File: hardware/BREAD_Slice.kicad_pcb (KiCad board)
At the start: 2 copper layers, 72.6 x 100 mm, 16 parts, among them J1 Conn_01x10_Female, J2 I2C_01x04

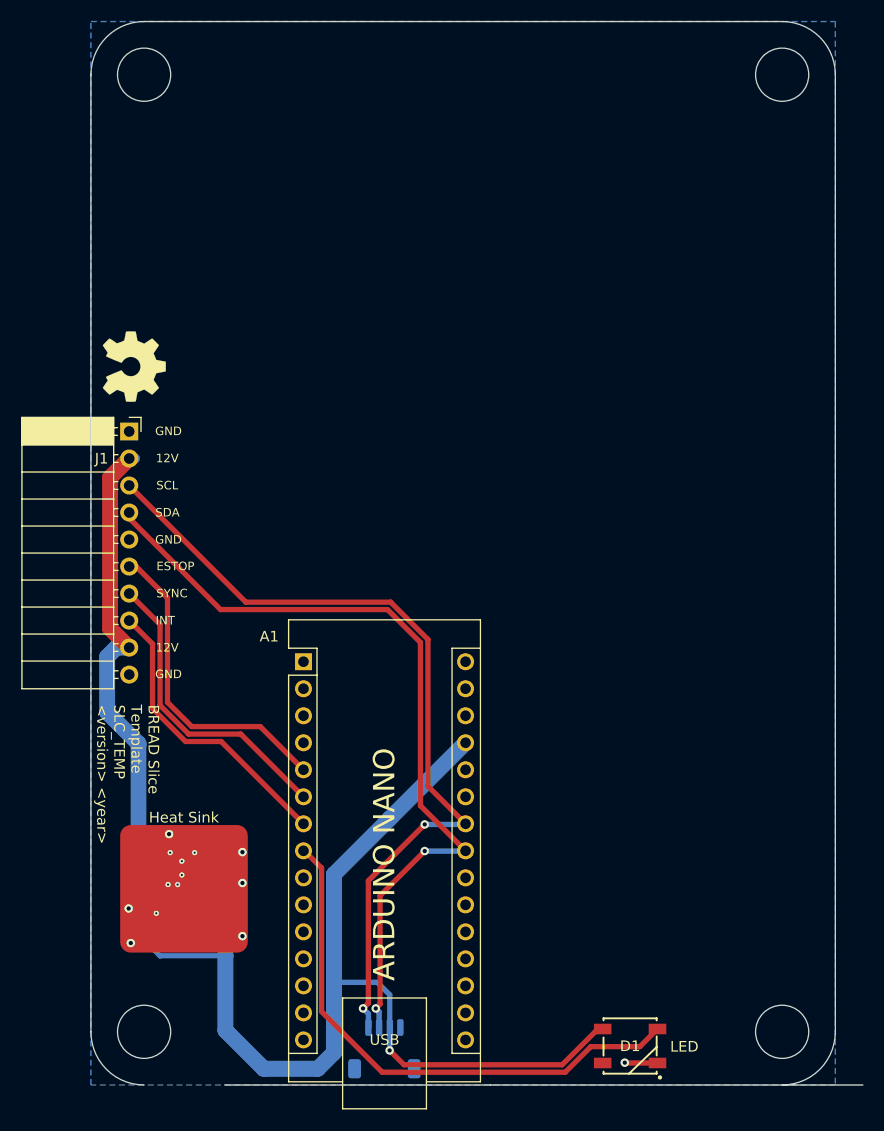
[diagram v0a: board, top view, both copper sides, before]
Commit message: Initial commit
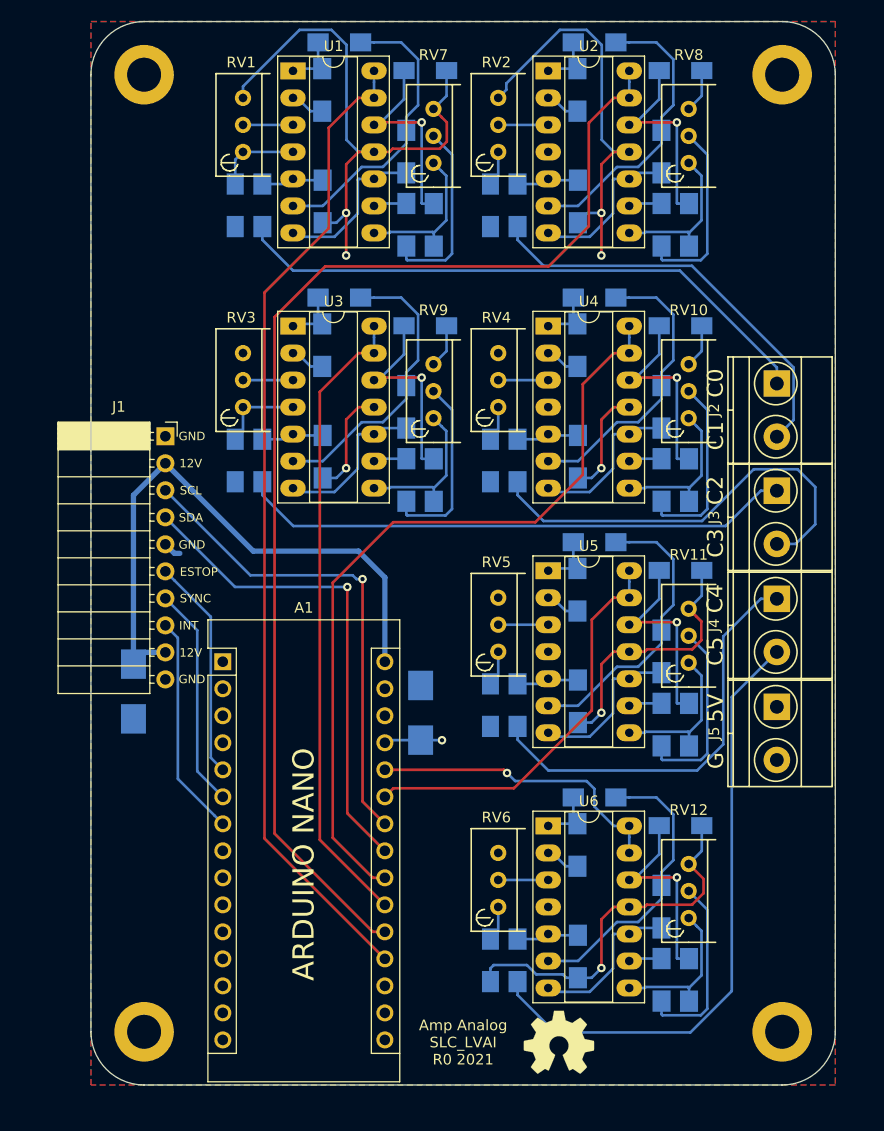
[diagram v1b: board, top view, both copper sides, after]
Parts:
- removed D1: WS2812B_5050, SparkFun-LED:WS2812-5050-4PIN
- removed HS1: Heatsink_Pad, SparkFun-Fuse:Thermal Pad
- removed L1: 4.7uH, Inductor_SMD:L_1210_3225Metric
- added C10: 1uF_t, OCI_UPL_FOOTPRINTS:C_1206_HandSoldering, B.Cu at (178.0, 44.4)
- added C11: 1uF_t, OCI_UPL_FOOTPRINTS:C_1206_HandSoldering, B.Cu at (154.0, 68.4)
- added C12: 1uF_t, OCI_UPL_FOOTPRINTS:C_1206_HandSoldering, B.Cu at (178.0, 68.4)
- added C13: 1uF_t, OCI_UPL_FOOTPRINTS:C_1206_HandSoldering, B.Cu at (178.0, 91.4)
- added C14: 1uF_t, OCI_UPL_FOOTPRINTS:C_1206_HandSoldering, B.Cu at (178.0, 115.4)
- added C5: 1uF_t, OCI_UPL_FOOTPRINTS:C_1206_HandSoldering, B.Cu at (136.2, 81.1)
- added C6: 1uF_t, OCI_UPL_FOOTPRINTS:C_1206_HandSoldering, B.Cu at (160.2, 81.1)
- added C7: 1uF_t, OCI_UPL_FOOTPRINTS:C_1206_HandSoldering, B.Cu at (160.2, 104.1)
- added C8: 1uF_t, OCI_UPL_FOOTPRINTS:C_1206_HandSoldering, B.Cu at (160.2, 128.1)
- added C9: 1uF_t, OCI_UPL_FOOTPRINTS:C_1206_HandSoldering, B.Cu at (154.0, 44.4)
- added J3: Term_2, OCI_UPL_FOOTPRINTS:TerminalBlock_Pheonix_MKDS1.5-2pol, F.Cu at (187.1, 83.9)
- added J4: Term_2, OCI_UPL_FOOTPRINTS:TerminalBlock_Pheonix_MKDS1.5-2pol, F.Cu at (187.1, 94.1)
- added J5: Term_2, OCI_UPL_FOOTPRINTS:TerminalBlock_Pheonix_MKDS1.5-2pol, F.Cu at (187.1, 104.2)
- added R1: 1K, OCI_UPL_FOOTPRINTS:R_1206_HandSoldering, B.Cu at (144.3, 46.2)
- added R10: 1K, OCI_UPL_FOOTPRINTS:R_1206_HandSoldering, B.Cu at (170.0, 41.8)
- added R11: 1K, OCI_UPL_FOOTPRINTS:R_1206_HandSoldering, B.Cu at (138.7, 81.1)
- added R12: 1K, OCI_UPL_FOOTPRINTS:R_1206_HandSoldering, B.Cu at (146.0, 65.8)
- added R13: 1K, OCI_UPL_FOOTPRINTS:R_1206_HandSoldering, B.Cu at (162.7, 81.1)
- added R14: 1K, OCI_UPL_FOOTPRINTS:R_1206_HandSoldering, B.Cu at (170.0, 65.8)
- added R15: 1K, OCI_UPL_FOOTPRINTS:R_1206_HandSoldering, B.Cu at (162.7, 104.1)
- added R16: 1K, OCI_UPL_FOOTPRINTS:R_1206_HandSoldering, B.Cu at (170.0, 88.8)
- added R17: 1K, OCI_UPL_FOOTPRINTS:R_1206_HandSoldering, B.Cu at (162.7, 128.1)
- added R18: 1K, OCI_UPL_FOOTPRINTS:R_1206_HandSoldering, B.Cu at (170.0, 112.8)
- added R19: 1K, OCI_UPL_FOOTPRINTS:R_1206_HandSoldering, B.Cu at (144.4, 56.7)
- added R2: 1K, OCI_UPL_FOOTPRINTS:R_1206_HandSoldering, B.Cu at (168.3, 46.2)
- added R20: 1K, OCI_UPL_FOOTPRINTS:R_1206_HandSoldering, B.Cu at (168.4, 56.7)
- added R21: 1K, OCI_UPL_FOOTPRINTS:R_1206_HandSoldering, B.Cu at (144.4, 80.7)
- added R22: 1K, OCI_UPL_FOOTPRINTS:R_1206_HandSoldering, B.Cu at (168.4, 80.7)
- added R23: 1K, OCI_UPL_FOOTPRINTS:R_1206_HandSoldering, B.Cu at (168.4, 103.7)
- added R24: 1K, OCI_UPL_FOOTPRINTS:R_1206_HandSoldering, B.Cu at (168.4, 127.7)
- added R25: 1K, OCI_UPL_FOOTPRINTS:R_1206_HandSoldering, B.Cu at (152.2, 52.0)
- added R26: 1K, OCI_UPL_FOOTPRINTS:R_1206_HandSoldering, B.Cu at (176.2, 52.0)
- added R27: 1K, OCI_UPL_FOOTPRINTS:R_1206_HandSoldering, B.Cu at (152.2, 76.0)
- added R28: 1K, OCI_UPL_FOOTPRINTS:R_1206_HandSoldering, B.Cu at (176.2, 76.0)
- added R29: 1K, OCI_UPL_FOOTPRINTS:R_1206_HandSoldering, B.Cu at (176.2, 99.0)
- added R3: 1K, OCI_UPL_FOOTPRINTS:R_1206_HandSoldering, B.Cu at (144.3, 70.2)
- added R30: 1K, OCI_UPL_FOOTPRINTS:R_1206_HandSoldering, B.Cu at (176.2, 123.0)
- added R31: 1K, OCI_UPL_FOOTPRINTS:R_1206_HandSoldering, B.Cu at (152.3, 58.9)
- added R32: 1K, OCI_UPL_FOOTPRINTS:R_1206_HandSoldering, B.Cu at (176.3, 58.9)
- added R33: 1K, OCI_UPL_FOOTPRINTS:R_1206_HandSoldering, B.Cu at (152.3, 82.9)
- added R34: 1K, OCI_UPL_FOOTPRINTS:R_1206_HandSoldering, B.Cu at (176.3, 82.9)
- added R35: 1K, OCI_UPL_FOOTPRINTS:R_1206_HandSoldering, B.Cu at (176.3, 105.9)
- added R36: 1K, OCI_UPL_FOOTPRINTS:R_1206_HandSoldering, B.Cu at (176.3, 129.9)
- added R37: 1K, OCI_UPL_FOOTPRINTS:R_1206_HandSoldering, B.Cu at (154.8, 58.9)
- added R38: 1K, OCI_UPL_FOOTPRINTS:R_1206_HandSoldering, B.Cu at (178.8, 58.9)
- added R39: 1K, OCI_UPL_FOOTPRINTS:R_1206_HandSoldering, B.Cu at (154.8, 82.9)
- added R4: 1K, OCI_UPL_FOOTPRINTS:R_1206_HandSoldering, B.Cu at (168.3, 70.2)
- added R40: 1K, OCI_UPL_FOOTPRINTS:R_1206_HandSoldering, B.Cu at (178.8, 82.9)
- added R41: 1K, OCI_UPL_FOOTPRINTS:R_1206_HandSoldering, B.Cu at (178.8, 105.9)
- added R42: 1K, OCI_UPL_FOOTPRINTS:R_1206_HandSoldering, B.Cu at (178.8, 129.9)
- added R5: 1K, OCI_UPL_FOOTPRINTS:R_1206_HandSoldering, B.Cu at (168.3, 93.2)
- added R6: 1K, OCI_UPL_FOOTPRINTS:R_1206_HandSoldering, B.Cu at (168.3, 117.2)
- added R7: 1K, OCI_UPL_FOOTPRINTS:R_1206_HandSoldering, B.Cu at (138.7, 57.1)
- added R8: 1K, OCI_UPL_FOOTPRINTS:R_1206_HandSoldering, B.Cu at (146.0, 41.8)
- added R9: 1K, OCI_UPL_FOOTPRINTS:R_1206_HandSoldering, B.Cu at (162.7, 57.1)
- added RV1: 10k_t, OCI_UPL_FOOTPRINTS:Potentiometer_Bourns_3296W_3-8Zoll_Inline_ScrewUp, F.Cu at (136.9, 52.1)
- added RV10: 10k_t, OCI_UPL_FOOTPRINTS:Potentiometer_Bourns_3296W_3-8Zoll_Inline_ScrewUp, F.Cu at (178.8, 77.1)
- added RV11: 10k_t, OCI_UPL_FOOTPRINTS:Potentiometer_Bourns_3296W_3-8Zoll_Inline_ScrewUp, F.Cu at (178.8, 100.1)
- added RV12: 10k_t, OCI_UPL_FOOTPRINTS:Potentiometer_Bourns_3296W_3-8Zoll_Inline_ScrewUp, F.Cu at (178.8, 124.1)
- added RV2: 10k_t, OCI_UPL_FOOTPRINTS:Potentiometer_Bourns_3296W_3-8Zoll_Inline_ScrewUp, F.Cu at (160.9, 52.1)
- added RV3: 10k_t, OCI_UPL_FOOTPRINTS:Potentiometer_Bourns_3296W_3-8Zoll_Inline_ScrewUp, F.Cu at (136.9, 76.1)
- added RV4: 10k_t, OCI_UPL_FOOTPRINTS:Potentiometer_Bourns_3296W_3-8Zoll_Inline_ScrewUp, F.Cu at (160.9, 76.1)
- added RV5: 10k_t, OCI_UPL_FOOTPRINTS:Potentiometer_Bourns_3296W_3-8Zoll_Inline_ScrewUp, F.Cu at (160.9, 99.1)
- added RV6: 10k_t, OCI_UPL_FOOTPRINTS:Potentiometer_Bourns_3296W_3-8Zoll_Inline_ScrewUp, F.Cu at (160.9, 123.1)
- added RV7: 10k_t, OCI_UPL_FOOTPRINTS:Potentiometer_Bourns_3296W_3-8Zoll_Inline_ScrewUp, F.Cu at (154.8, 53.1)
- added RV8: 10k_t, OCI_UPL_FOOTPRINTS:Potentiometer_Bourns_3296W_3-8Zoll_Inline_ScrewUp, F.Cu at (178.8, 53.1)
- added RV9: 10k_t, OCI_UPL_FOOTPRINTS:Potentiometer_Bourns_3296W_3-8Zoll_Inline_ScrewUp, F.Cu at (154.8, 77.1)
- added U2: MCP6004, Package_DIP:DIP-14_W7.62mm_Socket_LongPads, F.Cu at (165.6, 44.4)
- added U3: MCP6004, Package_DIP:DIP-14_W7.62mm_Socket_LongPads, F.Cu at (141.6, 68.4)
- added U4: MCP6004, Package_DIP:DIP-14_W7.62mm_Socket_LongPads, F.Cu at (165.6, 68.4)
- added U5: MCP6004, Package_DIP:DIP-14_W7.62mm_Socket_LongPads, F.Cu at (165.6, 91.4)
- added U6: MCP6004, Package_DIP:DIP-14_W7.62mm_Socket_LongPads, F.Cu at (165.6, 115.4)
- C1: value 22uF -> 10uF_t; footprint Capacitor_SMD:C_1206_3216Metric -> OCI_UPL_FOOTPRINTS:C_2312
- C2: value 100nF -> 10uF_t; footprint Capacitor_SMD:C_1206_3216Metric -> OCI_UPL_FOOTPRINTS:C_2312
- C3, C4: value 22uF -> 1uF_t; footprint Capacitor_SMD:C_1206_3216Metric -> OCI_UPL_FOOTPRINTS:C_1206_HandSoldering
- H1, H4: footprint MountingHole:MountingHole_5mm -> MountingHole:MountingHole_3.2mm_M3_DIN965_Pad
- H2: renamed from H3; footprint MountingHole:MountingHole_5mm -> MountingHole:MountingHole_3.2mm_M3_DIN965_Pad
- H3: renamed from H2; footprint MountingHole:MountingHole_5mm -> MountingHole:MountingHole_3.2mm_M3_DIN965_Pad
- J2: value I2C_01x04 -> Term_2; footprint Connector_JST:JST_SH_SM04B-SRSS-TB_1x04-1MP_P1.00mm_Horizontal -> OCI_UPL_FOOTPRINTS:TerminalBlock_Pheonix_MKDS1.5-2pol; moved to F.Cu
- U1: value ~ -> MCP6004; footprint Package_TO_SOT_SMD:TSOT-23-6 -> Package_DIP:DIP-14_W7.62mm_Socket_LongPads; moved to F.Cu
- moved U1 79.4 mm to (141.6, 44.4)
- moved Logo1 75.1 mm to (166.6, 135.8), turned to 0 degrees
- moved J2 72.6 mm to (187.1, 73.8), turned to -90 degrees
- moved C4 64.9 mm to (160.2, 57.1), turned to -90 degrees
- moved C3 62.4 mm to (136.2, 57.1), turned to -90 degrees
- moved C2 31.1 mm to (153.6, 104.8), turned to 90 degrees
- moved C1 16.8 mm to (126.6, 102.8), turned to -90 degrees
- moved A1 7.59 mm to (135.0, 100.0)
- moved J1 3.43 mm to (129.6, 78.8)
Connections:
- A1 pad 1: unconnected-(A1-D1/TX-Pad1) -> Net-(A1-Pad1)
- A1 pad 10: unconnected-(A1-D7-Pad10) -> Net-(A1-Pad10)
- A1 pad 11: unconnected-(A1-D8-Pad11) -> Net-(A1-Pad11)
- A1 pad 12: unconnected-(A1-D9-Pad12) -> Net-(A1-Pad12)
- A1 pad 13: unconnected-(A1-D10-Pad13) -> Net-(A1-Pad13)
- A1 pad 14: unconnected-(A1-D11-Pad14) -> Net-(A1-Pad14)
- A1 pad 15: unconnected-(A1-D12-Pad15) -> Net-(A1-Pad15)
- A1 pad 16: unconnected-(A1-D13-Pad16) -> Net-(A1-Pad16)
- A1 pad 17: unconnected-(A1-3V3-Pad17) -> Net-(A1-Pad17)
- A1 pad 18: unconnected-(A1-AREF-Pad18) -> Net-(A1-Pad18)
- A1 pad 19: unconnected-(A1-A0-Pad19) -> /CH0_AI
- A1 pad 2: unconnected-(A1-D0/RX-Pad2) -> Net-(A1-Pad2)
- A1 pad 20: unconnected-(A1-A1-Pad20) -> /CH1_AI
- A1 pad 21: unconnected-(A1-A2-Pad21) -> /CH2_AI
- A1 pad 22: unconnected-(A1-A3-Pad22) -> /CH3_AI
- A1 pad 25: unconnected-(A1-A6-Pad25) -> /CH4_AI
- A1 pad 26: unconnected-(A1-A7-Pad26) -> /CH5_AI
- A1 pad 28: unconnected-(A1-~{RESET}-Pad28) -> Net-(A1-Pad28)
- A1 pad 3: unconnected-(A1-~{RESET}-Pad3) -> Net-(A1-Pad3)
- A1 pad 30: unconnected-(A1-VIN-Pad30) -> +12V
- A1 pad 6: /INT -> /SYNC
- A1 pad 7: /SYNC -> /INT
- A1 pad 8: /LED -> Net-(A1-Pad8)
- A1 pad 9: unconnected-(A1-D6-Pad9) -> Net-(A1-Pad9)
- C1 pad 1: GND -> +12V
- C1 pad 2: +12V -> GND
- C2 pad 1: Net-(U1-SW) -> +5V
- C2 pad 2: Net-(U1-BST) -> GND
- C3 pad 1: GND -> +5V
- C3 pad 2: +5V -> GND
- C4 pad 1: GND -> +5V
- C4 pad 2: +5V -> GND
- J1 pad 7: /INT -> /SYNC
- J1 pad 8: /SYNC -> /INT
- J2 pad 1: GND -> /Ch0_in
- J2 pad 2: +5V -> /Ch1_in
- U1 pad 1: +5V -> Net-(R1-Pad2)
- U1 pad 2: +12V -> Net-(R1-Pad1)
- U1 pad 3: +12V -> Net-(RV1-Pad2)
- U1 pad 4: GND -> +5V
- U1 pad 5: Net-(U1-SW) -> Net-(R19-Pad2)
- U1 pad 6: Net-(U1-BST) -> Net-(R25-Pad1)
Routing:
- net GND: track 19.6 -> 189.4 mm, vias 14 -> 8
- net /CH1_AI: track 0.00 -> 112.9 mm
- net /CH0_AI: track 0.00 -> 93.3 mm
- net /CH3_AI: track 0.00 -> 74.8 mm
- net +5V: track 108.9 -> 34.8 mm
- net /CH2_AI: track 0.00 -> 59.9 mm
- net /Ch5_in: track 0.00 -> 58.1 mm
- net /Ch0_in: track 0.00 -> 56.1 mm
- net /Ch2_in: track 0.00 -> 52.2 mm
- net /LED: track 51.5 -> 0.00 mm
- net /Ch3_in: track 0.00 -> 40.8 mm
- net /Ch4_in: track 0.00 -> 39.5 mm
- net /Ch1_in: track 0.00 -> 39.3 mm
- net /CH4_AI: track 0.00 -> 38.3 mm
- net /I2C_CLK: track 78.5 -> 45.9 mm, vias 2 -> 1
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- added copper zone on F.Cu, net +5V
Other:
- board size 72.6 x 100 mm -> 70 x 100 mm
- board text added: "5V"
- board text added: "Amp Analog SLC_LVAI R0 2021"
- board text added: "C0"
- board text added: "C1"
- board text added: "C2"
- board text added: "C3"
- board text added: "C4"
- board text added: "C5"
- board text added: "G"
- board text removed: "12V->5V Reg"
- board text removed: "5V I2C Connector"
- board text removed: "BREAD Slice Template SLC_TEMP <version> <year>"
- board text removed: "LED"

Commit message: extensive documentation, remade board, subcircuits for all
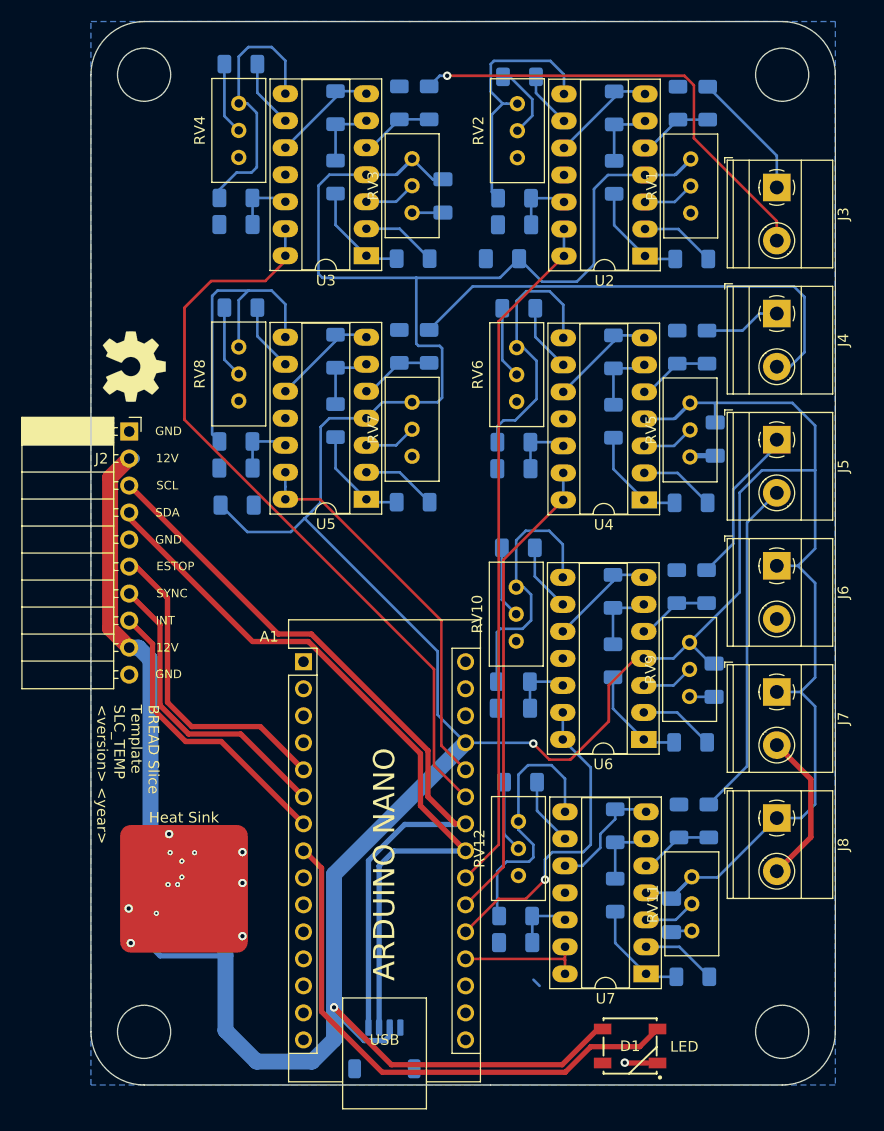
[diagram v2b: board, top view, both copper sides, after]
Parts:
- removed the J2 at (187.1, 73.8)
- added C15: 1uF_t, Capacitor_SMD:C_1206_3216Metric_Pad1.33x1.80mm_HandSolder, B.Cu at (177.2, 123.9)
- added C16: 1uF_t, Capacitor_SMD:C_1206_3216Metric_Pad1.33x1.80mm_HandSolder, B.Cu at (162.5, 126.4)
- added D1: WS2812B_5050, SparkFun-LED:WS2812-5050-4PIN, F.Cu at (173.3, 136.1)
- added HS1: Heatsink_Pad, KML-Custom:Thermal Pad, F.Cu at (131.3, 121.4)
- added J1: I2C_01x04, Connector_JST:JST_SH_SM04B-SRSS-TB_1x04-1MP_P1.00mm_Horizontal, B.Cu at (150.2, 136.4)
- added J6: Term_2, TerminalBlock_Phoenix:TerminalBlock_Phoenix_MKDS-1,5-2_1x02_P5.00mm_Horizontal, F.Cu at (187.1, 91.0)
- added J7: Term_2, TerminalBlock_Phoenix:TerminalBlock_Phoenix_MKDS-1,5-2_1x02_P5.00mm_Horizontal, F.Cu at (187.1, 102.8)
- added J8: Term_2, TerminalBlock_Phoenix:TerminalBlock_Phoenix_MKDS-1,5-2_1x02_P5.00mm_Horizontal, F.Cu at (187.1, 114.7)
- added L1: 4.7uH, Inductor_SMD:L_1210_3225Metric, B.Cu at (133.8, 122.8)
- added U7: MCP6004, Package_DIP:DIP-14_W7.62mm_Socket_LongPads, F.Cu at (174.8, 129.3)
- C1: value 10uF_t -> 22uF; footprint OCI_UPL_FOOTPRINTS:C_2312 -> Capacitor_SMD:C_1206_3216Metric
- C10, C11, C12, C13, C14, C5, C6, C7, C8, C9: footprint OCI_UPL_FOOTPRINTS:C_1206_HandSoldering -> Capacitor_SMD:C_1206_3216Metric_Pad1.33x1.80mm_HandSolder
- C2: value 10uF_t -> 100nF; footprint OCI_UPL_FOOTPRINTS:C_2312 -> Capacitor_SMD:C_1206_3216Metric
- C3, C4: value 1uF_t -> 22uF; footprint OCI_UPL_FOOTPRINTS:C_1206_HandSoldering -> Capacitor_SMD:C_1206_3216Metric
- H1, H4: footprint MountingHole:MountingHole_3.2mm_M3_DIN965_Pad -> MountingHole:MountingHole_5mm
- H2: renamed from H3; footprint MountingHole:MountingHole_3.2mm_M3_DIN965_Pad -> MountingHole:MountingHole_5mm
- H3: renamed from H2; footprint MountingHole:MountingHole_3.2mm_M3_DIN965_Pad -> MountingHole:MountingHole_5mm
- J3, J4, J5: footprint OCI_UPL_FOOTPRINTS:TerminalBlock_Pheonix_MKDS1.5-2pol -> TerminalBlock_Phoenix:TerminalBlock_Phoenix_MKDS-1,5-2_1x02_P5.00mm_Horizontal
- R1, R10, R11, R12, R13, R14, R15, R16, R17, R18, R19, R2, R20, R21, R22, R23, R24, R25, R26, R27, R28, R29, R3, R30, R31, R32, R33, R34, R35, R36, R37, R38, R39, R4, R40, R41, R42, R5, R6, R7, R8, R9: footprint OCI_UPL_FOOTPRINTS:R_1206_HandSoldering -> Resistor_SMD:R_1206_3216Metric_Pad1.30x1.75mm_HandSolder
- RV1, RV10, RV11, RV12, RV2, RV3, RV4, RV5, RV6, RV7, RV8, RV9: footprint OCI_UPL_FOOTPRINTS:Potentiometer_Bourns_3296W_3-8Zoll_Inline_ScrewUp -> Potentiometer_THT:Potentiometer_Bourns_3296W_Vertical
- U1: value MCP6004 -> ~; footprint Package_DIP:DIP-14_W7.62mm_Socket_LongPads -> Package_TO_SOT_SMD:TSOT-23-6; moved to B.Cu
- moved U1 79.4 mm to (128.8, 122.8)
- moved Logo1 75.1 mm to (126.7, 72.2), turned to -90 degrees
- moved C8 73.2 mm to (136.2, 58.9), turned to 180 degrees
- moved R6 72.4 mm to (162.9, 45.0), turned to 180 degrees
- moved C4 64.9 mm to (133.8, 116.5), turned to 0 degrees
- moved R38 63.4 mm to (171.9, 122.0)
- moved C3 62.4 mm to (133.8, 119.5), turned to 0 degrees
- moved R37 61.7 mm to (180.7, 115.0), turned to -90 degrees
- moved R24 55.3 mm to (145.6, 77.3)
- moved RV6 52.6 mm to (162.6, 70.5), turned to 90 degrees
- moved R17 51.5 mm to (171.7, 77.4)
- moved C7 48.1 mm to (155.7, 56.2)
- moved RV8 45.7 mm to (136.5, 70.4), turned to 90 degrees
- moved R13 45.5 mm to (136.7, 43.8), turned to 180 degrees
- moved R5 45.4 mm to (171.8, 47.9)
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- renumbered J1 to J2
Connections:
- A1 pad 1: Net-(A1-Pad1) -> unconnected-(A1-D1/TX-Pad1)
- A1 pad 10: Net-(A1-Pad10) -> unconnected-(A1-D7-Pad10)
- A1 pad 11: Net-(A1-Pad11) -> unconnected-(A1-D8-Pad11)
- A1 pad 12: Net-(A1-Pad12) -> unconnected-(A1-D9-Pad12)
- A1 pad 13: Net-(A1-Pad13) -> unconnected-(A1-D10-Pad13)
- A1 pad 14: Net-(A1-Pad14) -> unconnected-(A1-D11-Pad14)
- A1 pad 15: Net-(A1-Pad15) -> unconnected-(A1-D12-Pad15)
- A1 pad 16: Net-(A1-Pad16) -> unconnected-(A1-D13-Pad16)
- A1 pad 17: Net-(A1-Pad17) -> unconnected-(A1-3V3-Pad17)
- A1 pad 18: Net-(A1-Pad18) -> unconnected-(A1-AREF-Pad18)
- A1 pad 19: /CH0_AI -> /CH5_AI
- A1 pad 2: Net-(A1-Pad2) -> unconnected-(A1-D0/RX-Pad2)
- A1 pad 20: /CH1_AI -> /CH4_AI
- A1 pad 22: /CH3_AI -> /CH0_AI
- A1 pad 25: /CH4_AI -> /CH1_AI
- A1 pad 26: /CH5_AI -> /CH3_AI
- A1 pad 28: Net-(A1-Pad28) -> unconnected-(A1-~{RESET}-Pad28)
- A1 pad 3: Net-(A1-Pad3) -> unconnected-(A1-~{RESET}-Pad3)
- A1 pad 30: +12V -> unconnected-(A1-VIN-Pad30)
- A1 pad 6: /SYNC -> /INT
- A1 pad 7: /INT -> /SYNC
- A1 pad 8: Net-(A1-Pad8) -> /LED
- A1 pad 9: Net-(A1-Pad9) -> unconnected-(A1-D6-Pad9)
- C1 pad 1: +12V -> GND
- C1 pad 2: GND -> +12V
- C10 pad 1: Net-(C10-Pad1) -> Net-(U4D-+)
- C11 pad 1: Net-(C11-Pad1) -> +5V
- C12 pad 1: Net-(C12-Pad1) -> Net-(U5D-+)
- C13 pad 1: Net-(C13-Pad1) -> +5V
- C14 pad 1: Net-(C14-Pad1) -> Net-(U6D-+)
- C2 pad 1: +5V -> Net-(U1-SW)
- C2 pad 2: GND -> Net-(U1-BST)
- C3 pad 1: +5V -> GND
- C3 pad 2: GND -> +5V
- C4 pad 1: +5V -> GND
- C4 pad 2: GND -> +5V
- C6 pad 1: +5V -> Net-(U2D-+)
- C8 pad 1: +5V -> Net-(U3D-+)
- C9 pad 1: Net-(C9-Pad1) -> +5V
- J2 pad 7: /SYNC -> /INT
- J2 pad 8: /INT -> /SYNC
- J3 pad 1: /Ch2_in -> /Ch0_in
- J3 pad 2: /Ch3_in -> /Ch1_in
- J4 pad 1: /Ch4_in -> /Ch2_in
- J4 pad 2: /Ch5_in -> /Ch3_in
- J5 pad 1: +5V -> /Ch4_in
- J5 pad 2: GND -> /Ch5_in
- R1 pad 1: Net-(R1-Pad1) -> Net-(U2A--)
- R10 pad 2: Net-(R10-Pad2) -> Net-(U3B--)
- R11 pad 1: /Ch2_in -> GND
- R11 pad 2: Net-(R11-Pad2) -> Net-(U3B-+)
- R12 pad 1: Net-(R12-Pad1) -> Net-(U3B--)
- R12 pad 2: Net-(R12-Pad2) -> Net-(U3C-+)
- R13 pad 1: /Ch3_in -> Net-(U3C--)
- R14 pad 2: Net-(R14-Pad2) -> Net-(U3D-+)
- R15 pad 1: /Ch4_in -> Net-(U4A--)
- R16 pad 1: Net-(R16-Pad1) -> /Ch2_in
- R16 pad 2: Net-(R16-Pad2) -> Net-(U4B-+)
- R17 pad 1: /Ch5_in -> Net-(R15-Pad2)
- R17 pad 2: Net-(R17-Pad2) -> Net-(U4B--)
- R18 pad 1: Net-(R18-Pad1) -> GND
- R18 pad 2: Net-(R18-Pad2) -> Net-(U4B-+)
- R19 pad 1: GND -> Net-(U4B--)
- R19 pad 2: Net-(R19-Pad2) -> Net-(U4C-+)
- R2 pad 1: Net-(R2-Pad1) -> /Ch0_in
- R2 pad 2: Net-(R10-Pad1) -> Net-(U2B-+)
- R20 pad 1: GND -> Net-(U4C--)
- R21 pad 1: GND -> Net-(R21-Pad1)
- R21 pad 2: Net-(R11-Pad2) -> Net-(U4D-+)
- R22 pad 1: GND -> Net-(U5A--)
- R22 pad 2: Net-(R13-Pad2) -> Net-(R22-Pad2)
- R23 pad 1: GND -> /Ch3_in
- R23 pad 2: Net-(R15-Pad2) -> Net-(U5B-+)
- R24 pad 1: GND -> Net-(R22-Pad2)
- R24 pad 2: Net-(R17-Pad2) -> Net-(U5B--)
- R25 pad 1: Net-(R25-Pad1) -> GND
- R25 pad 2: Net-(R25-Pad2) -> Net-(U5B-+)
- R26 pad 1: Net-(R10-Pad2) -> Net-(U5B--)
- R26 pad 2: Net-(R26-Pad2) -> Net-(U5C-+)
- R27 pad 1: Net-(R12-Pad2) -> Net-(U5C--)
- R28 pad 1: Net-(R14-Pad2) -> Net-(R28-Pad1)
- R28 pad 2: Net-(R28-Pad2) -> Net-(U5D-+)
- R29 pad 1: Net-(R16-Pad2) -> Net-(U6A--)
- R3 pad 1: Net-(R3-Pad1) -> Net-(R1-Pad2)
- R3 pad 2: Net-(R12-Pad1) -> Net-(U2B--)
- R30 pad 1: Net-(R18-Pad2) -> /Ch4_in
- R30 pad 2: Net-(R30-Pad2) -> Net-(U6B-+)
- R31 pad 1: Net-(R31-Pad1) -> Net-(R29-Pad2)
- R31 pad 2: Net-(R31-Pad2) -> Net-(U6B--)
- R32 pad 1: Net-(R32-Pad1) -> GND
- R32 pad 2: Net-(R32-Pad2) -> Net-(U6B-+)
- R33 pad 1: Net-(R33-Pad1) -> Net-(U6B--)
- R33 pad 2: Net-(R33-Pad2) -> Net-(U6C-+)
- R34 pad 1: Net-(R34-Pad1) -> Net-(U6C--)
- R35 pad 2: Net-(R35-Pad2) -> Net-(U6D-+)
- R36 pad 1: Net-(R36-Pad1) -> Net-(U7A--)
- R37 pad 1: Net-(R37-Pad1) -> /Ch5_in
- R37 pad 2: Net-(C9-Pad1) -> Net-(U7B-+)
- R38 pad 1: Net-(R38-Pad1) -> Net-(R36-Pad2)
- R38 pad 2: Net-(C10-Pad1) -> Net-(U7B--)
- R39 pad 1: Net-(R39-Pad1) -> GND
- R39 pad 2: Net-(C11-Pad1) -> Net-(U7B-+)
- R4 pad 1: Net-(R4-Pad1) -> GND
- R4 pad 2: Net-(R14-Pad1) -> Net-(U2B-+)
- R40 pad 1: Net-(R40-Pad1) -> Net-(U7B--)
- R40 pad 2: Net-(C12-Pad1) -> Net-(U7C-+)
- R41 pad 1: Net-(R41-Pad1) -> Net-(U7C--)
- R41 pad 2: Net-(C13-Pad1) -> Net-(R41-Pad2)
- R42 pad 2: Net-(C14-Pad1) -> Net-(U7D-+)
- R5 pad 1: Net-(R5-Pad1) -> Net-(U2B--)
- R5 pad 2: Net-(R16-Pad1) -> Net-(U2C-+)
- R6 pad 1: Net-(R6-Pad1) -> Net-(U2C--)
- R6 pad 2: Net-(R18-Pad1) -> Net-(R6-Pad2)
- R7 pad 1: /Ch0_in -> Net-(R7-Pad1)
- R7 pad 2: Net-(R19-Pad2) -> Net-(U2D-+)
- R8 pad 1: Net-(R1-Pad2) -> Net-(U3A--)
- R8 pad 2: Net-(R25-Pad1) -> Net-(R10-Pad1)
- R9 pad 2: Net-(R20-Pad2) -> Net-(U3B-+)
- RV1 pad 2: Net-(RV1-Pad2) -> Net-(U2A-+)
- RV10 pad 1: Net-(R40-Pad1) -> Net-(R35-Pad1)
- RV11 pad 1: Net-(R41-Pad1) -> +5V
- RV11 pad 2: Net-(R35-Pad2) -> Net-(U7A-+)
- RV12 pad 2: Net-(R36-Pad2) -> Net-(R41-Pad2)
- RV2 pad 1: +5V -> Net-(R7-Pad1)
- RV2 pad 2: Net-(RV2-Pad2) -> Net-(R6-Pad2)
- RV4 pad 1: +5V -> Net-(R14-Pad1)
- RV4 pad 2: Net-(RV4-Pad2) -> Net-(R13-Pad2)
- RV5 pad 2: Net-(RV5-Pad2) -> Net-(U4A-+)
- RV6 pad 1: +5V -> Net-(R21-Pad1)
- RV6 pad 2: Net-(RV6-Pad2) -> Net-(R20-Pad2)
- RV7 pad 1: Net-(R37-Pad1) -> +5V
- RV7 pad 2: Net-(R31-Pad2) -> Net-(U5A-+)
- RV8 pad 1: Net-(R38-Pad1) -> Net-(R28-Pad1)
- RV8 pad 2: Net-(R32-Pad2) -> Net-(R27-Pad2)
- RV9 pad 1: Net-(R39-Pad1) -> +5V
- RV9 pad 2: Net-(R33-Pad2) -> Net-(U6A-+)
- U1 pad 1: Net-(R1-Pad2) -> +5V
- U1 pad 2: Net-(R1-Pad1) -> +12V
- U1 pad 3: Net-(RV1-Pad2) -> +12V
- U1 pad 4: +5V -> GND
- U1 pad 5: Net-(R19-Pad2) -> Net-(U1-SW)
- U1 pad 6: Net-(R25-Pad1) -> Net-(U1-BST)
- U2 pad 1: Net-(R10-Pad1) -> Net-(R1-Pad2)
- U2 pad 10: Net-(R26-Pad2) -> Net-(U2C-+)
- U2 pad 12: Net-(C10-Pad1) -> Net-(U2D-+)
- U2 pad 13: /CH1_AI -> /CH0_AI
- U2 pad 14: /CH1_AI -> /CH0_AI
- U2 pad 2: Net-(R2-Pad1) -> Net-(U2A--)
- U2 pad 3: Net-(RV2-Pad2) -> Net-(U2A-+)
- U2 pad 5: Net-(R20-Pad2) -> Net-(U2B-+)
- U2 pad 6: Net-(R10-Pad2) -> Net-(U2B--)
- U2 pad 7: Net-(R26-Pad2) -> Net-(U2C-+)
- U2 pad 8: Net-(R38-Pad1) -> Net-(R7-Pad1)
- U2 pad 9: Net-(R32-Pad1) -> Net-(U2C--)
- U3 pad 1: Net-(R12-Pad1) -> Net-(R10-Pad1)
- U3 pad 10: Net-(R27-Pad2) -> Net-(U3C-+)
- U3 pad 12: Net-(C11-Pad1) -> Net-(U3D-+)
- U3 pad 13: /CH2_AI -> /CH1_AI
- U3 pad 14: /CH2_AI -> /CH1_AI
- U3 pad 2: Net-(R3-Pad1) -> Net-(U3A--)
- U3 pad 5: Net-(R11-Pad2) -> Net-(U3B-+)
- U3 pad 6: Net-(R12-Pad2) -> Net-(U3B--)
- U3 pad 7: Net-(R27-Pad2) -> Net-(U3C-+)
- U3 pad 8: Net-(R39-Pad1) -> Net-(R14-Pad1)
- U3 pad 9: Net-(R33-Pad1) -> Net-(U3C--)
- U4 pad 1: Net-(R14-Pad1) -> Net-(R15-Pad2)
- U4 pad 10: Net-(R28-Pad2) -> Net-(U4C-+)
- U4 pad 12: Net-(C12-Pad1) -> Net-(U4D-+)
- U4 pad 13: /CH3_AI -> /CH2_AI
- U4 pad 14: /CH3_AI -> /CH2_AI
- U4 pad 2: Net-(R4-Pad1) -> Net-(U4A--)
- U4 pad 3: Net-(RV4-Pad2) -> Net-(U4A-+)
- U4 pad 5: Net-(R13-Pad2) -> Net-(U4B-+)
- U4 pad 6: Net-(R14-Pad2) -> Net-(U4B--)
- U4 pad 7: Net-(R28-Pad2) -> Net-(U4C-+)
- U4 pad 8: Net-(R40-Pad1) -> Net-(R21-Pad1)
- U4 pad 9: Net-(R34-Pad1) -> Net-(U4C--)
- U5 pad 1: Net-(R16-Pad1) -> Net-(R22-Pad2)
- U5 pad 10: Net-(R29-Pad2) -> Net-(U5C-+)
- U5 pad 12: Net-(C13-Pad1) -> Net-(U5D-+)
- U5 pad 13: /CH4_AI -> /CH3_AI
- U5 pad 14: /CH4_AI -> /CH3_AI
- U5 pad 2: Net-(R5-Pad1) -> Net-(U5A--)
- U5 pad 3: Net-(RV5-Pad2) -> Net-(U5A-+)
- U5 pad 5: Net-(R15-Pad2) -> Net-(U5B-+)
- U5 pad 6: Net-(R16-Pad2) -> Net-(U5B--)
- U5 pad 7: Net-(R29-Pad2) -> Net-(U5C-+)
- U5 pad 8: Net-(R41-Pad1) -> Net-(R28-Pad1)
- U5 pad 9: Net-(R35-Pad1) -> Net-(U5C--)
- U6 pad 1: Net-(R18-Pad1) -> Net-(R29-Pad2)
- U6 pad 10: Net-(R30-Pad2) -> Net-(U6C-+)
- U6 pad 12: Net-(C14-Pad1) -> Net-(U6D-+)
- U6 pad 13: /CH5_AI -> /CH4_AI
- U6 pad 14: /CH5_AI -> /CH4_AI
- U6 pad 2: Net-(R6-Pad1) -> Net-(U6A--)
- U6 pad 3: Net-(RV6-Pad2) -> Net-(U6A-+)
- U6 pad 5: Net-(R17-Pad2) -> Net-(U6B-+)
- U6 pad 6: Net-(R18-Pad2) -> Net-(U6B--)
- U6 pad 7: Net-(R30-Pad2) -> Net-(U6C-+)
- U6 pad 8: Net-(R42-Pad1) -> Net-(R35-Pad1)
- U6 pad 9: Net-(R36-Pad1) -> Net-(U6C--)
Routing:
- net +5V: track 34.8 -> 397.4 mm, vias 1 -> 2
- net GND: track 189.4 -> 32.0 mm, vias 8 -> 14
- net /LED: track 0.00 -> 51.5 mm
- net /Ch2_in: track 52.2 -> 7.22 mm
- net /Ch0_in: track 56.1 -> 12.2 mm
- net /CH1_AI: track 112.9 -> 71.3 mm
- net /CH3_AI: track 74.8 -> 36.9 mm
- net Net-(R28-Pad1): track 0.00 -> 30.4 mm
- net /CH0_AI: track 93.3 -> 64.8 mm
- net /I2C_CLK: track 45.9 -> 73.6 mm, vias 1 -> 0
- net Net-(R25-Pad1): track 27.5 -> 0.00 mm
- net Net-(R10-Pad2): track 27.5 -> 0.00 mm
- net Net-(R16-Pad2): track 27.5 -> 0.00 mm
- net Net-(R14-Pad2): track 27.5 -> 0.00 mm
- net Net-(R12-Pad2): track 27.5 -> 0.00 mm
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- removed copper zone on F.Cu, net +5V
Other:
- outline, holes or cut-outs redrawn
- board text added: "12V->5V Reg"
- board text added: "5V I2C Connector"
- board text added: "BREAD Slice Template SLC_TEMP <version> <year>"
- board text added: "LED"
- board text removed: "5V"
- board text removed: "Amp Analog SLC_LVAI R0 2021"
- board text removed: "C0"
- board text removed: "C1"
- board text removed: "C2"
- board text removed: "C3"
- board text removed: "C4"
- board text removed: "C5"
- board text removed: "G"
